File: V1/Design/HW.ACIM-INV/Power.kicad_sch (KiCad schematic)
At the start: 13 parts, among them J1 HIGH VOLT, J2 LOW VOLT

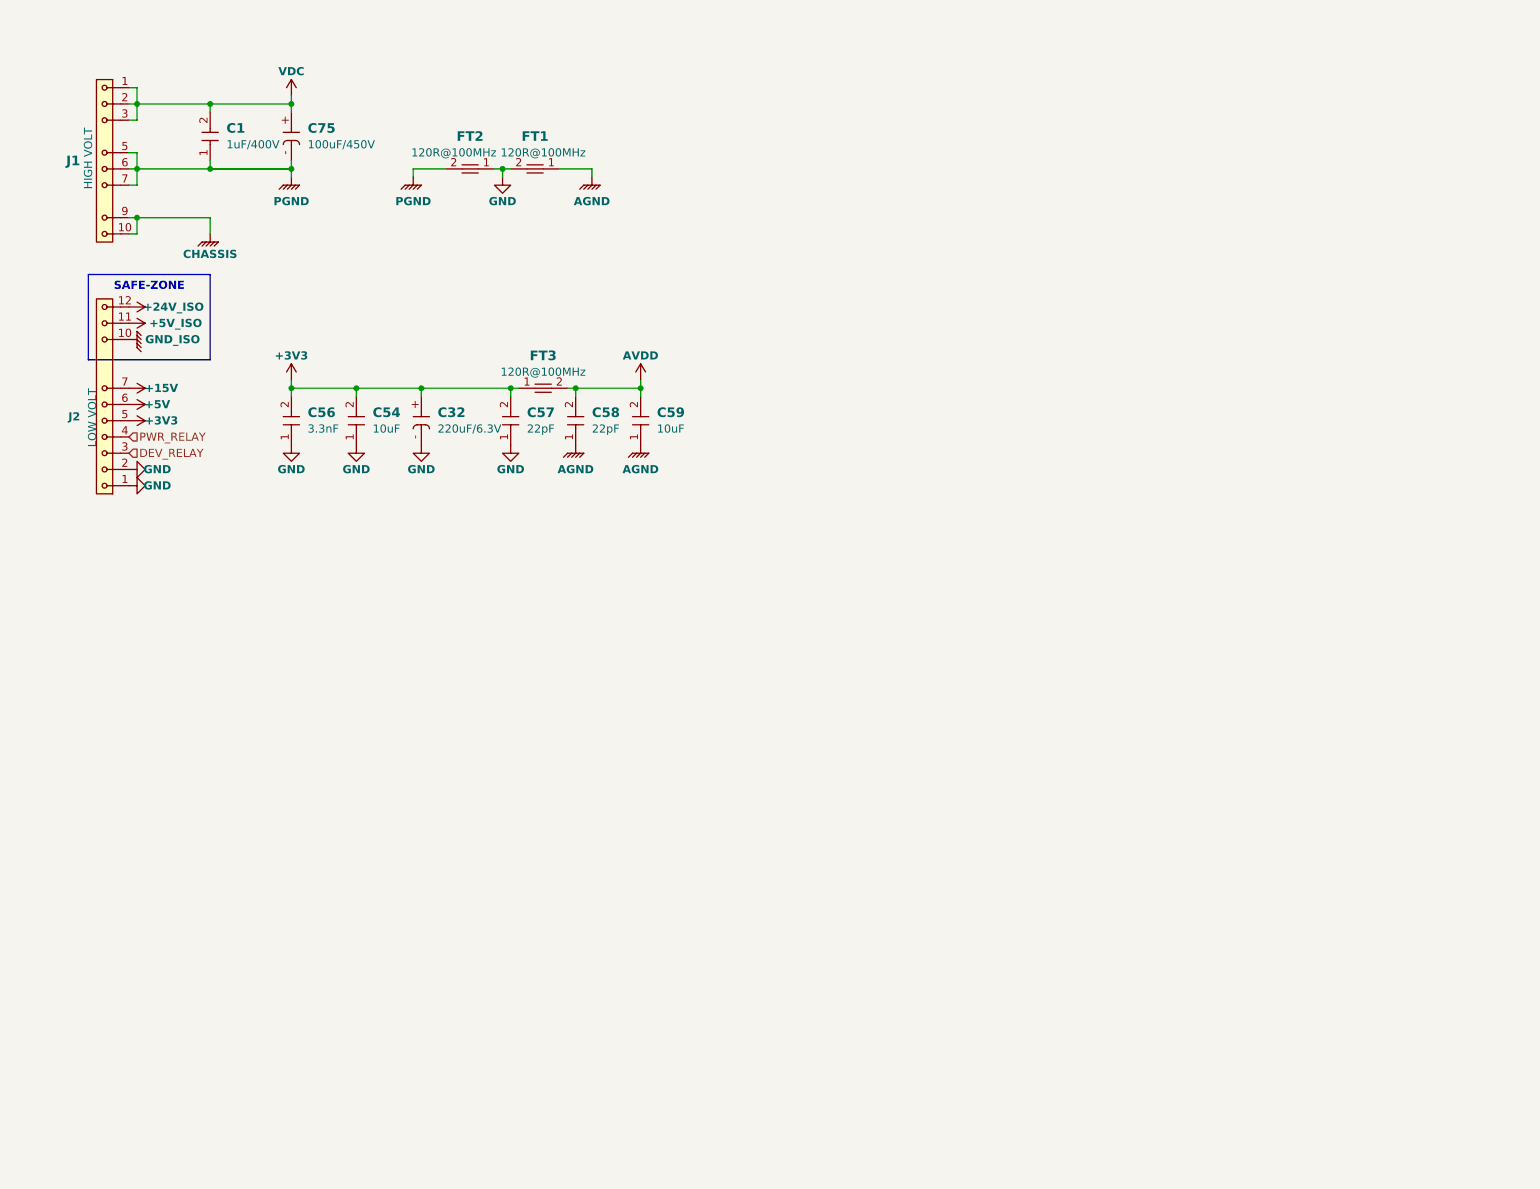
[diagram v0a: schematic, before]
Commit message: V1 schematic update 5
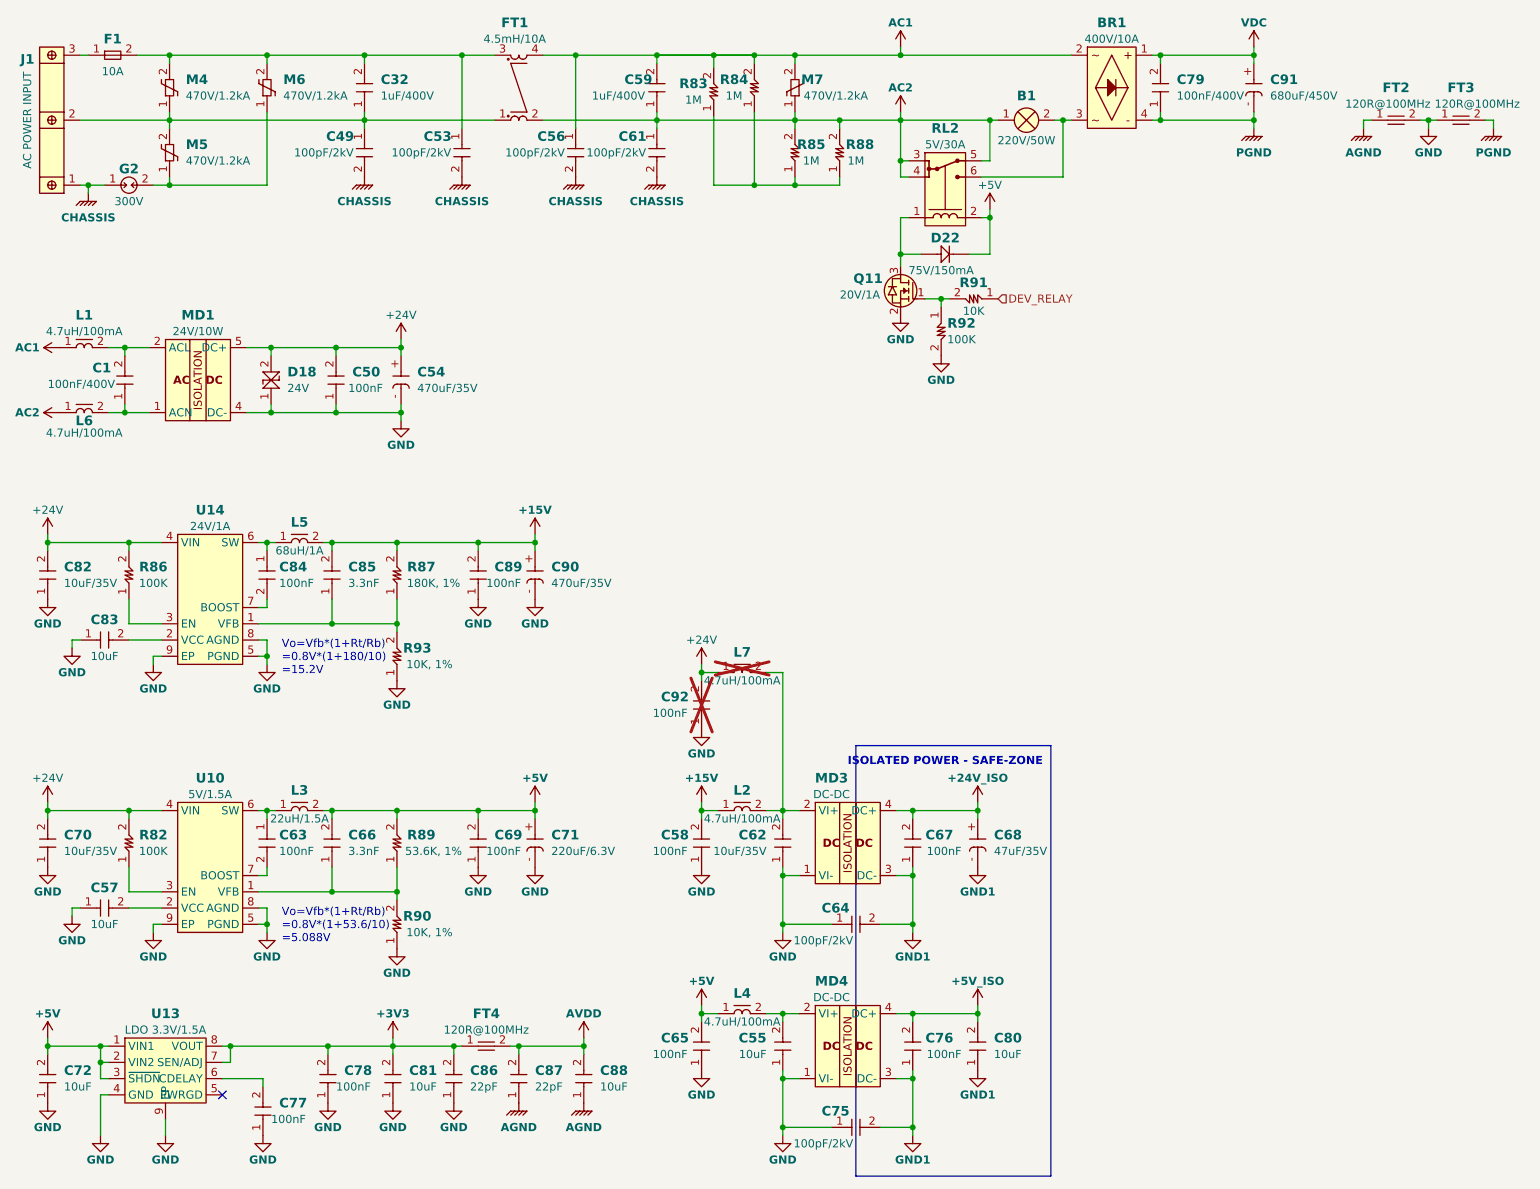
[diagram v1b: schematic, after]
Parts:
- removed C32: 220uF/6.3V, SAMPI:CAP1411, symbol SAMPI:ELECCAP
- removed C54: 10uF, SAMPI:CAP0603, symbol SAMPI:CERCAP
- removed C75: 100uF/450V, SAMPI:CAP_ELEC-18.0x51.5-LS7.5, symbol SAMPI:ELECCAP
- removed FT1: 120R@100MHz, SAMPI:FT0603, symbol SAMPI:FerriteBead
- removed J1: HIGH VOLT, SAMPI:HDM1x10x2.54_TH_RA, symbol SAMPI:SIL10
- removed J2: LOW VOLT, SAMPI:HDM1x12x2.54_TH_RA, symbol SAMPI:SIL12
- added B1: 220V/50W, SAMPI:LAMP_6.35MM, symbol SAMPI:Lamp
- added BR1: 400V/10A, SAMPI:GBJ25xx, symbol SAMPI:BRIDGE
- added C32: 1uF/400V, SAMPI:ECWFE2W105, symbol SAMPI:CERCAP
- added C49, C53, C61, C64, C75: 100pF/2kV, SAMPI:CAP1206, symbol SAMPI:CERCAP
- added C50, C63, C65, C67, C69, C76, C77, C78, C84, C89, C92: 100nF, SAMPI:CAP0603, symbol SAMPI:CERCAP
- added C54, C90: 470uF/35V, SAMPI:CAP_ELEC-10.3x10.3-DIA10, symbol SAMPI:ELECCAP
- added C55, C72, C80, C81, C83, C88: 10uF, SAMPI:CAP0603, symbol SAMPI:CERCAP
- added C62, C70, C82: 10uF/35V, SAMPI:CAP0603, symbol SAMPI:CERCAP
- added C66, C85: 3.3nF, SAMPI:CAP0603, symbol SAMPI:CERCAP
- added C68: 47uF/35V, SAMPI:CAP_ELEC-6.6x6.6-DIA6.3, symbol SAMPI:ELECCAP
- added C71: 220uF/6.3V, SAMPI:CAP1411, symbol SAMPI:ELECCAP
- added C79: 100nF/400V, SAMPI:CAP_FILM_6.0x12.0x12.5-P10, symbol SAMPI:CERCAP
- added C86, C87: 22pF, SAMPI:CAP0603, symbol SAMPI:CERCAP
- added C91: 680uF/450V, SAMPI:ESMQ451VSN681MA50S, symbol SAMPI:ELECCAP
- added D18: 24V, SAMPI:DO-214AA, symbol SAMPI:DIODE-TVS
- added D22: 75V/150mA, SAMPI:SOD-323, symbol SAMPI:DIODE-REC
- added F1: 10A, SAMPI:01000056Z, symbol SAMPI:FUSE
- added FT1: 4.5mH/10A, SAMPI:ToroidCoil-3119-13-D1, symbol SAMPI:CK_Choke_2
- added FT4: 120R@100MHz, SAMPI:FT0603, symbol SAMPI:FerriteBead
- added G2: 300V, SAMPI:GDT1812_3532, symbol SAMPI:GDT
- added J1: AC POWER INPUT, SAMPI:TMB3_9.5, symbol SAMPI:SIL03
- added L1, L2, L4, L6, L7: 4.7uH/100mA, SAMPI:IND0805, symbol SAMPI:IND
- added L3: 22uH/1.5A, SAMPI:IND6045, symbol SAMPI:IND
- added L5: 68uH/1A, SAMPI:IND6045, symbol SAMPI:IND
- added M4, M5, M6, M7: 470V/1.2kA, SAMPI:MOV5MM, symbol SAMPI:MOV
- added MD1: 24V/10W, SAMPI:LD10-23BxxR2-RC, symbol SAMPI:AC-DC
- added MD3, MD4: DC-DC, SAMPI:B1524S-1WR3, symbol SAMPI:DC-DC
- added Q11: 20V/1A, SAMPI:SOT23, symbol SAMPI:FET_N-CH
- added R82, R86, R92: 100K, SAMPI:RES0603, symbol SAMPI:RES
- added R83, R84, R85, R88: 1M, SAMPI:RES1206, symbol SAMPI:RES
- added R87: 180K, 1%, SAMPI:RES0603, symbol SAMPI:RES
- added R89: 53.6K, 1%, SAMPI:RES0603, symbol SAMPI:RES
- added R90, R93: 10K, 1%, SAMPI:RES0603, symbol SAMPI:RES
- added R91: 10K, SAMPI:RES0603, symbol SAMPI:RES
- added RL2: 5V/30A, SAMPI:SLA-12VDC-SL-C, symbol SAMPI:RELAY-SPST-6P
- added U10: 5V/1.5A, SAMPI:TDFN8_2x3_MCHP, symbol SAMPI:MCP16311-TDFN
- added U13: LDO 3.3V/1.5A, SAMPI:DFN8_3x3_MCHP, symbol SAMPI:MCP1727
- added U14: 24V/1A, SAMPI:TDFN8_2x3_MCHP, symbol SAMPI:MCP16311-TDFN
- C1: value 1uF/400V -> 100nF/400V; footprint SAMPI:ECWFE2W105 -> SAMPI:CAP_FILM_6.0x12.0x12.5-P10; MFT Panasonic -> VISHAY; MNP ECW-FE2W105K -> BFC233824104; Unit Price 0.72 -> 1.5
- C56: value 3.3nF -> 100pF/2kV; footprint SAMPI:CAP0603 -> SAMPI:CAP1206; MFT Samsung -> WE; MNP CL10B332KB8NNNC -> 885342208022; Unit Price 0.031 -> 0.19
- C57: value 22pF -> 10uF; MFT Walsin -> Samsung; MNP 0603N220J500CT -> CL10A106MQ8NNNC; Unit Price 0.012 -> 0.079
- C58: value 22pF -> 100nF; MFT Walsin -> Samsung; MNP 0603N220J500CT -> CL10B104KB8NNNC; Unit Price 0.012 -> 0.0146
- C59: value 10uF -> 1uF/400V; footprint SAMPI:CAP0603 -> SAMPI:ECWFE2W105; MFT Samsung -> Panasonic; MNP CL10A106MQ8NNNC -> ECW-FE2W105K; Unit Price 0.079 -> 0.72
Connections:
- net +15V: now also C58.2, C85.2, C89.2, C90.+, L2.1, L5.2, R87.2
- net +24V_ISO: now also C67.2, C68.+, MD3.4 (DC+)
- net +3V3: now also C78.2, C81.2, C86.2, FT4.1, U13.7 (SEN/ADJ), U13.8 (VOUT); no longer C56.2, C57.2, FT3.1
- net +5V: now also C65.2, C66.2, C69.2, C71.+, C72.2, D22.K, L3.2, L4.1, R89.2, RL2.2 (COIL2), U13.1 (VIN1), U13.2 (VIN2), U13.3 (~{SHDN})
- net +5V_ISO: now also C76.2, C80.2, MD4.4 (DC+)
- net AGND: now also FT2.1, C87.1, C88.1; no longer C58.1, C59.1
- net AVDD: now also C87.2, C88.2, FT4.2; no longer C58.2, C59.2, FT3.2
- net CHASSIS: now also C56.2, C49.2, C53.2, C61.2, G2.1, J1.1
- net DEV_RELAY: now also R91.1
- net GND: now also C58.1, FT2.2, FT3.1, C50.1, C54.-, C55.1, C62.1, C64.1, C65.1, C69.1, C70.1, C71.-, C72.1, C75.1, C77.1, C78.1, C81.1, C82.1, C83.1, C86.1, C89.1, C90.-, C92.1, D18.1 (A1), MD1.4 (DC-), MD3.1 (VI-), MD4.1 (VI-), Q11.2 (S), R90.1, R92.2, R93.1, U10.5 (PGND), U10.8 (AGND), U10.9 (EP), U13.4 (GND), U13.9 (EP), U14.5 (PGND), U14.8 (AGND), U14.9 (EP); no longer C56.1, FT2.1
- net PGND: now also FT3.2, BR1.4 (DC-), C79.1, C91.-; no longer C1.1, FT2.2
- net VDC: now also BR1.1 (DC+), C79.2, C91.+; no longer C1.2
- new net: R83.1, R84.1, R85.1, R88.1
- new net: G2.2, M5.1, M6.1
- new net: C83.2, U14.2 (VCC)
- new net: C84.1, L5.1, U14.6 (SW)
- new net: C32.2, C53.1, F1.2, FT1.3, M4.2, M6.2
- new net: C84.2, U14.7 (BOOST)
- new net: C32.1, C49.1, FT1.1, J1.2, M4.1, M5.2
- new net: C77.2, U13.6 (CDELAY)
- new net: D22.A, Q11.3 (D), RL2.1 (COIL1)
- new net: B1.2, BR1.3 (AC2), RL2.6 (NO)
- new net: C55.2, L4.2, MD4.2 (VI+)
- new net: C62.2, L2.2, L7.2, MD3.2 (VI+)
- new net: C1.2, L1.2, MD1.2 (ACL)
- new net: C85.1, R87.1, R93.2, U14.1 (VFB)
- new net: C66.1, R89.1, R90.2, U10.1 (VFB)
- new net: C63.1, L3.1, U10.6 (SW)
- new net: C57.2, U10.2 (VCC)
- new net: R82.1, U10.3 (EN)
- new net: C63.2, U10.7 (BOOST)
- new net: F1.1, J1.3
- new net: R86.1, U14.3 (EN)
- new net: Q11.1 (G), R91.2, R92.1
- new net: C1.1, L6.2, MD1.1 (ACN)
- new net +24V: C50.2, C54.+, C70.2, C82.2, C92.2, D18.2 (A2), L7.1, MD1.5 (DC+), R82.2, R86.2, U10.4 (VIN), U14.4 (VIN)
- new net AC1: BR1.2 (AC1), C56.1, C59.2, FT1.4, L1.1, M7.2, R83.2, R84.2
- new net AC2: B1.1, C59.1, C61.1, FT1.2, L6.1, M7.1, R85.2, R88.2, RL2.3 (COM), RL2.4 (COM), RL2.5 (NC)
- new net GND1: C64.2, C67.1, C68.-, C75.2, C76.1, C80.1, MD3.3 (DC-), MD4.3 (DC-)
- no-connect marks 0 -> 1
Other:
- note added: "ISOLATED POWER - SAFE-ZONE"
- note removed: "SAFE-ZONE"
